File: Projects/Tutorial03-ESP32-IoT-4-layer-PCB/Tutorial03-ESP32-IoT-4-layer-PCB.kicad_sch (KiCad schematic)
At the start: 19 parts, among them J1 SS-52400-002, J2 B2B-PH-SM4-TB, U1 MCP73871

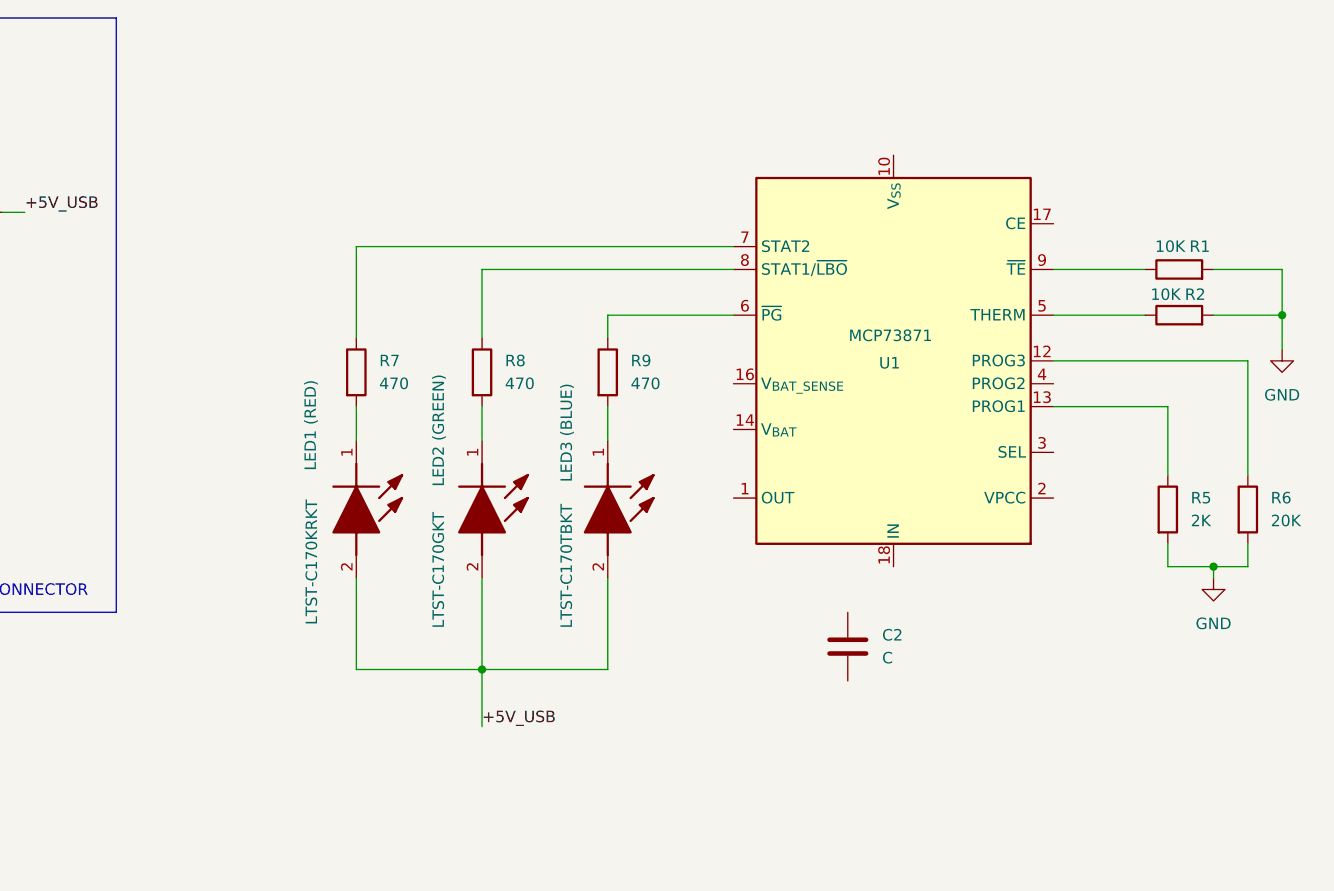
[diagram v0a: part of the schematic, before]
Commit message: 20260214
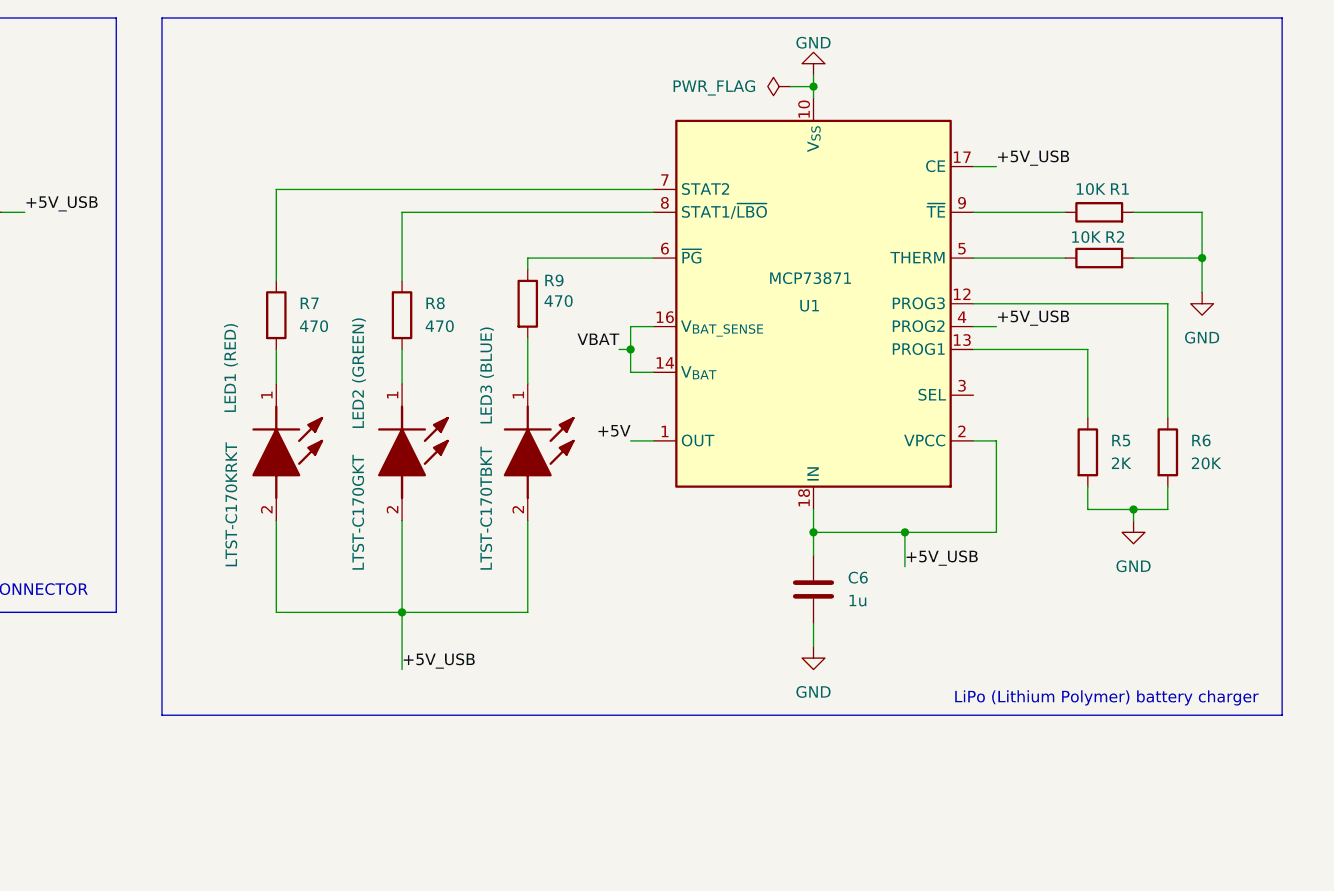
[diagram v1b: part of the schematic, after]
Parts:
- C6: renamed from C2; value C -> 1u
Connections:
- net +5V_USB: now also C6.1, U1.17 (CE), U1.18 (IN), U1.19 (IN), U1.2 (VPCC), U1.4 (PROG2)
- net GND: now also C6.2, U1.10 (V_{SS}), U1.11 (V_{SS}), U1.21 (V_{SS})
- net +5V: now reaches U1.1 (OUT), U1.20 (OUT)
- net VBAT: now reaches U1.14 (V_{BAT}), U1.15 (V_{BAT})
- net VBAT: now also U1.16 (V_{BAT_SENSE})
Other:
- note added: "LiPo (Lithium Polymer) battery charger"
- moved on the sheet: C6, LED1 (RED), LED2 (GREEN), LED3 (BLUE), R1, R2, R5, R6, R7, R8, R9, U1
